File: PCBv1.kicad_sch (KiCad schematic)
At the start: 20 parts, among them J1 AVR-ISP-6, SW2 SW_Push_Reset, U1 ATmega32U4-A, Y1 16MHz

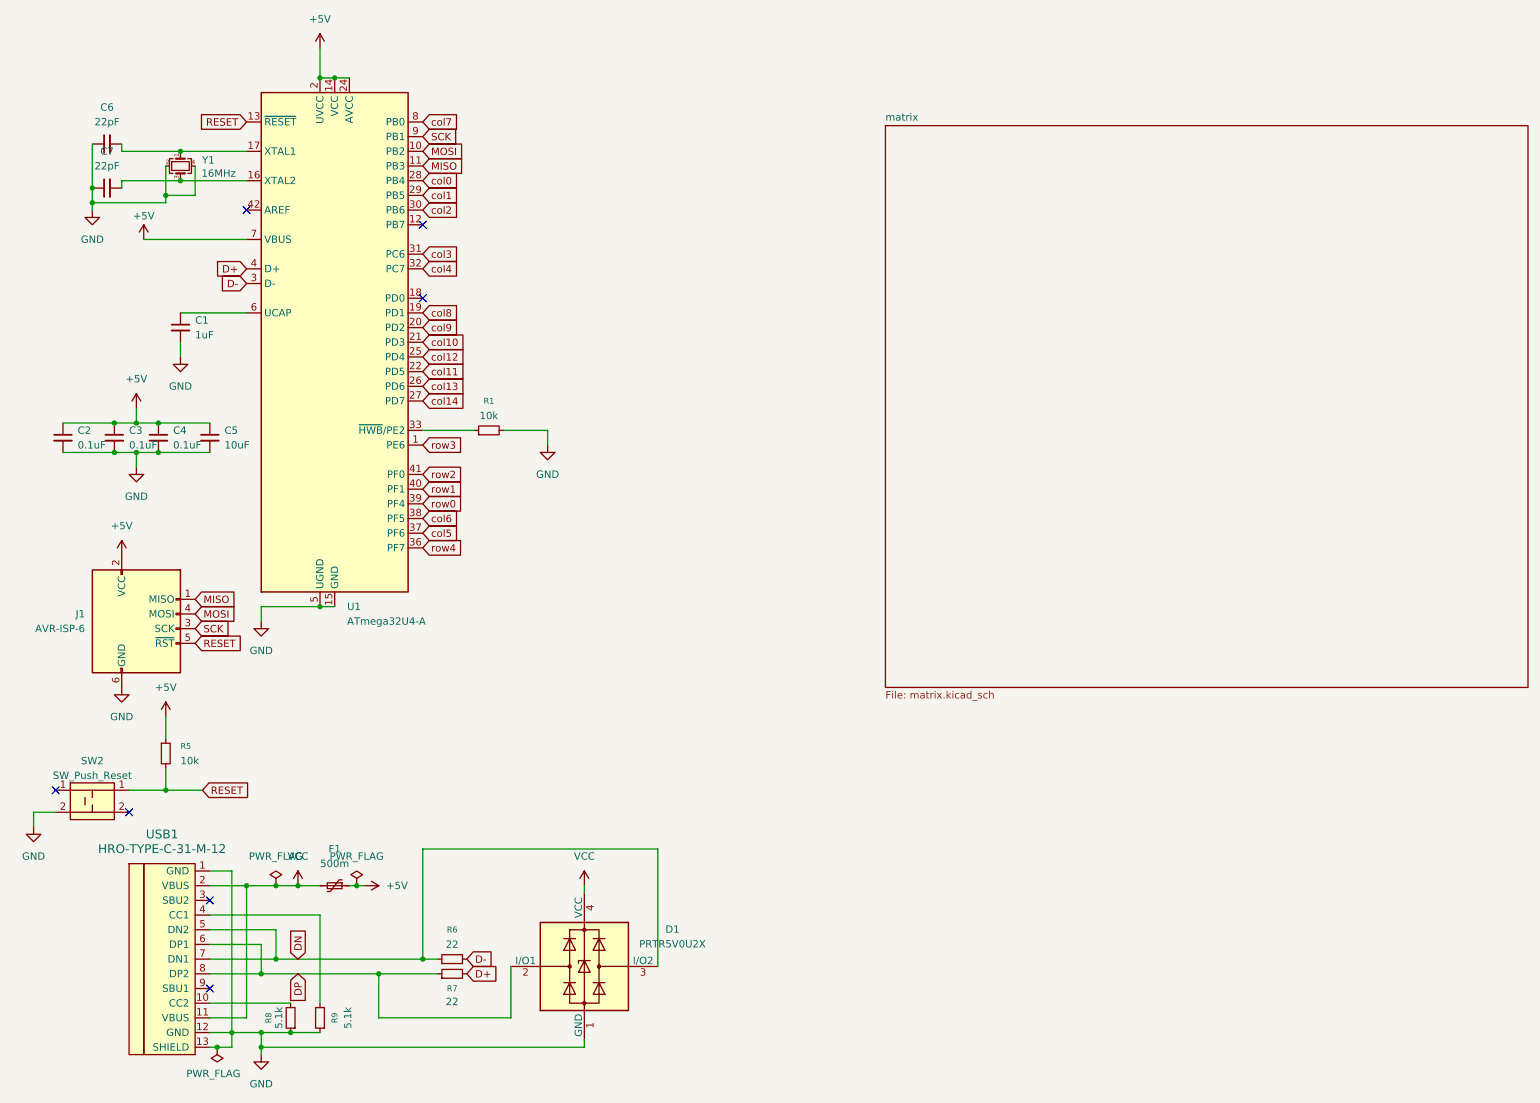
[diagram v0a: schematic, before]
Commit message: locked in
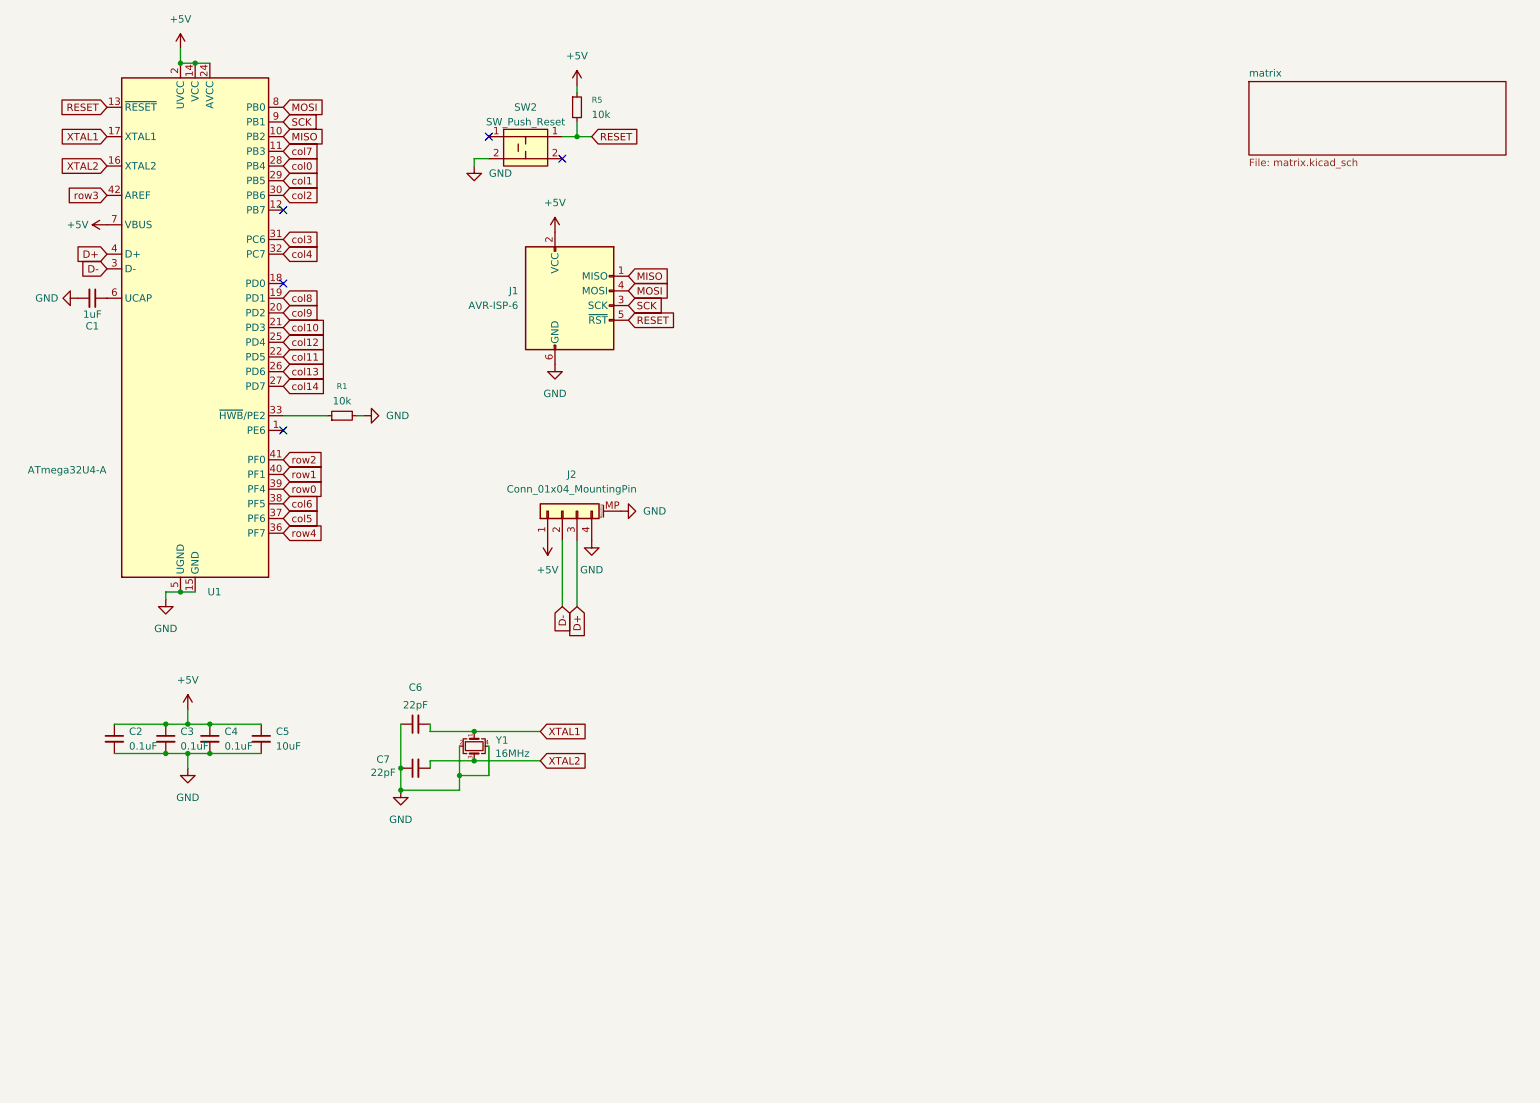
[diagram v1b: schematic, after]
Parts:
- removed D1: PRTR5V0U2X, Package_TO_SOT_SMD:SOT-143, symbol Power_Protection:PRTR5V0U2X
- removed F1: 500m, Fuse:Fuse_1206_3216Metric_Pad1.42x1.75mm_HandSolder, symbol Device:Polyfuse_Small
- removed R6, R7: 22, Resistor_SMD:R_0805_2012Metric_Pad1.20x1.40mm_HandSolder, symbol Device:R_Small
- removed R8, R9: 5.1k, Resistor_SMD:R_0805_2012Metric_Pad1.20x1.40mm_HandSolder, symbol Device:R_Small
- removed USB1: HRO-TYPE-C-31-M-12, Type-C:HRO-TYPE-C-31-M-12-HandSoldering, symbol Type-C:HRO-TYPE-C-31-M-12
- added J2: Conn_01x04_MountingPin, Connector_JST:JST_SH_SM04B-SRSS-TB_1x04-1MP_P1.00mm_Horizontal, symbol Connector_Generic_MountingPin:Conn_01x04_MountingPin
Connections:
- net +5V: now also J2.1 (Pin_1)
- net D+: now also J2.3 (Pin_3)
- net D-: now also J2.2 (Pin_2)
- net GND: now also J2.4 (Pin_4), J2.MP (MountPin)
- net MISO: now also U1.10 (PB2); no longer U1.11 (PB3)
- net MOSI: now also U1.8 (PB0); no longer U1.10 (PB2)
- net col7: now also U1.11 (PB3); no longer U1.8 (PB0)
- net row3: now also U1.42 (AREF); no longer U1.1 (PE6)
- net XTAL2: now reaches C7.2, U1.16 (XTAL2), Y1.3
- net XTAL1: now reaches C6.2, U1.17 (XTAL1), Y1.1
- no-connect marks 7 -> 5
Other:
- moved on the sheet: C1, C2, C3, C4, C5, C6, C7, J1, R1, R5, SW2, U1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
